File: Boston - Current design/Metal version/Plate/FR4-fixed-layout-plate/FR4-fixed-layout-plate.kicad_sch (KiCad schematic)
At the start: 14 parts

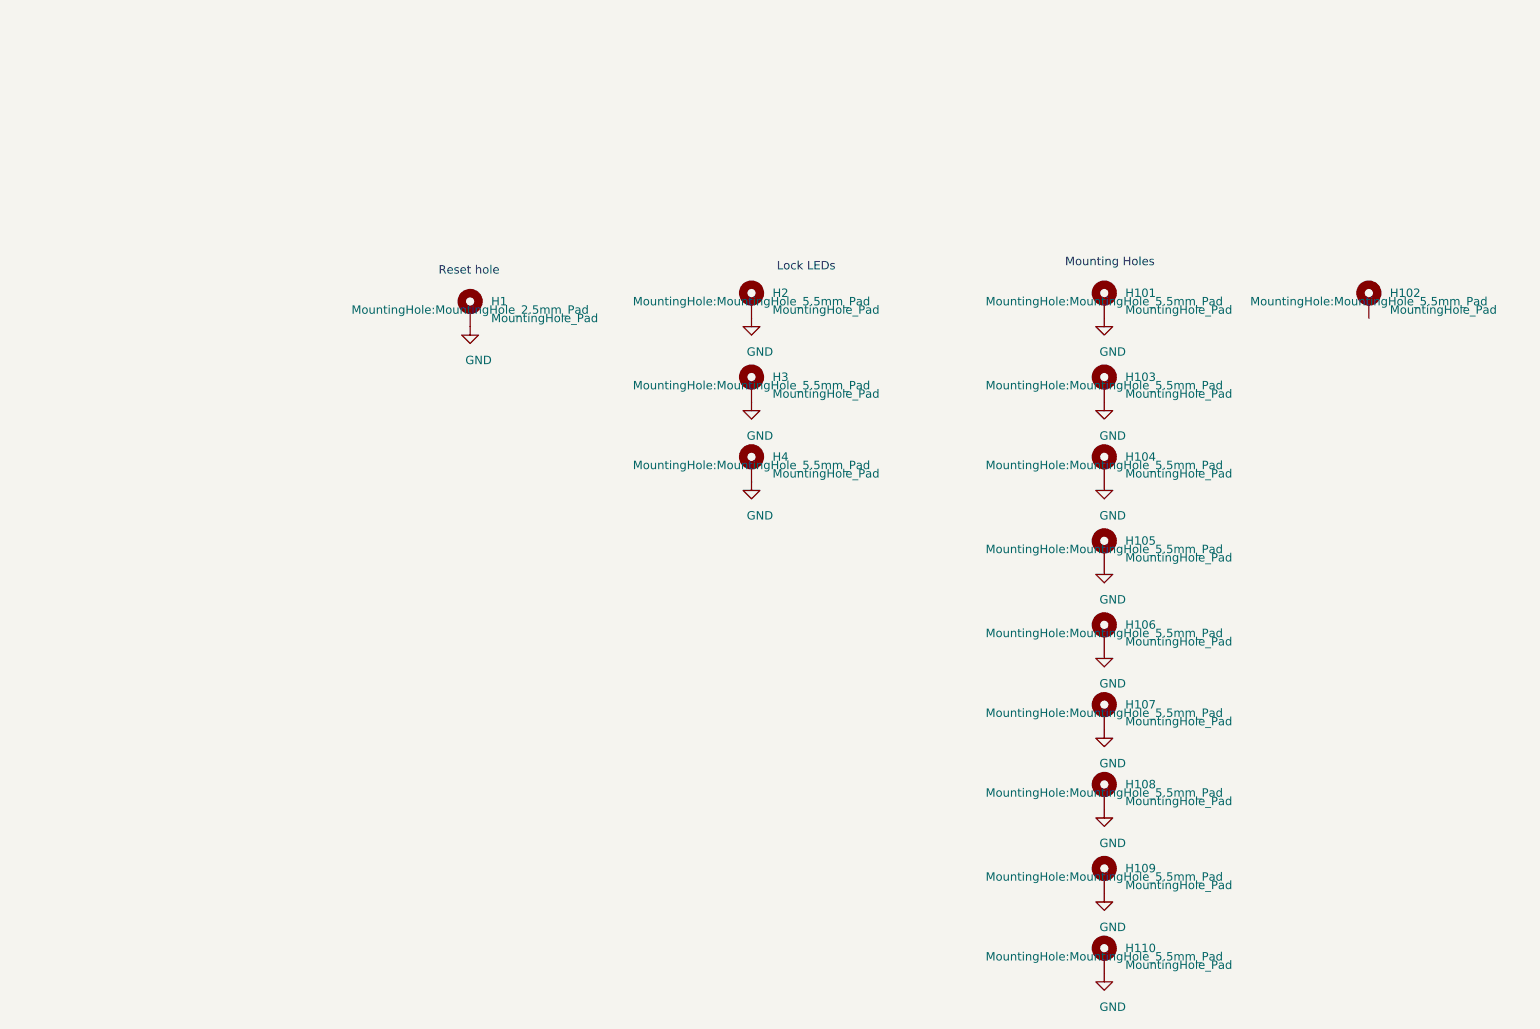
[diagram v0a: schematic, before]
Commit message: Finished work on fixed layout plate
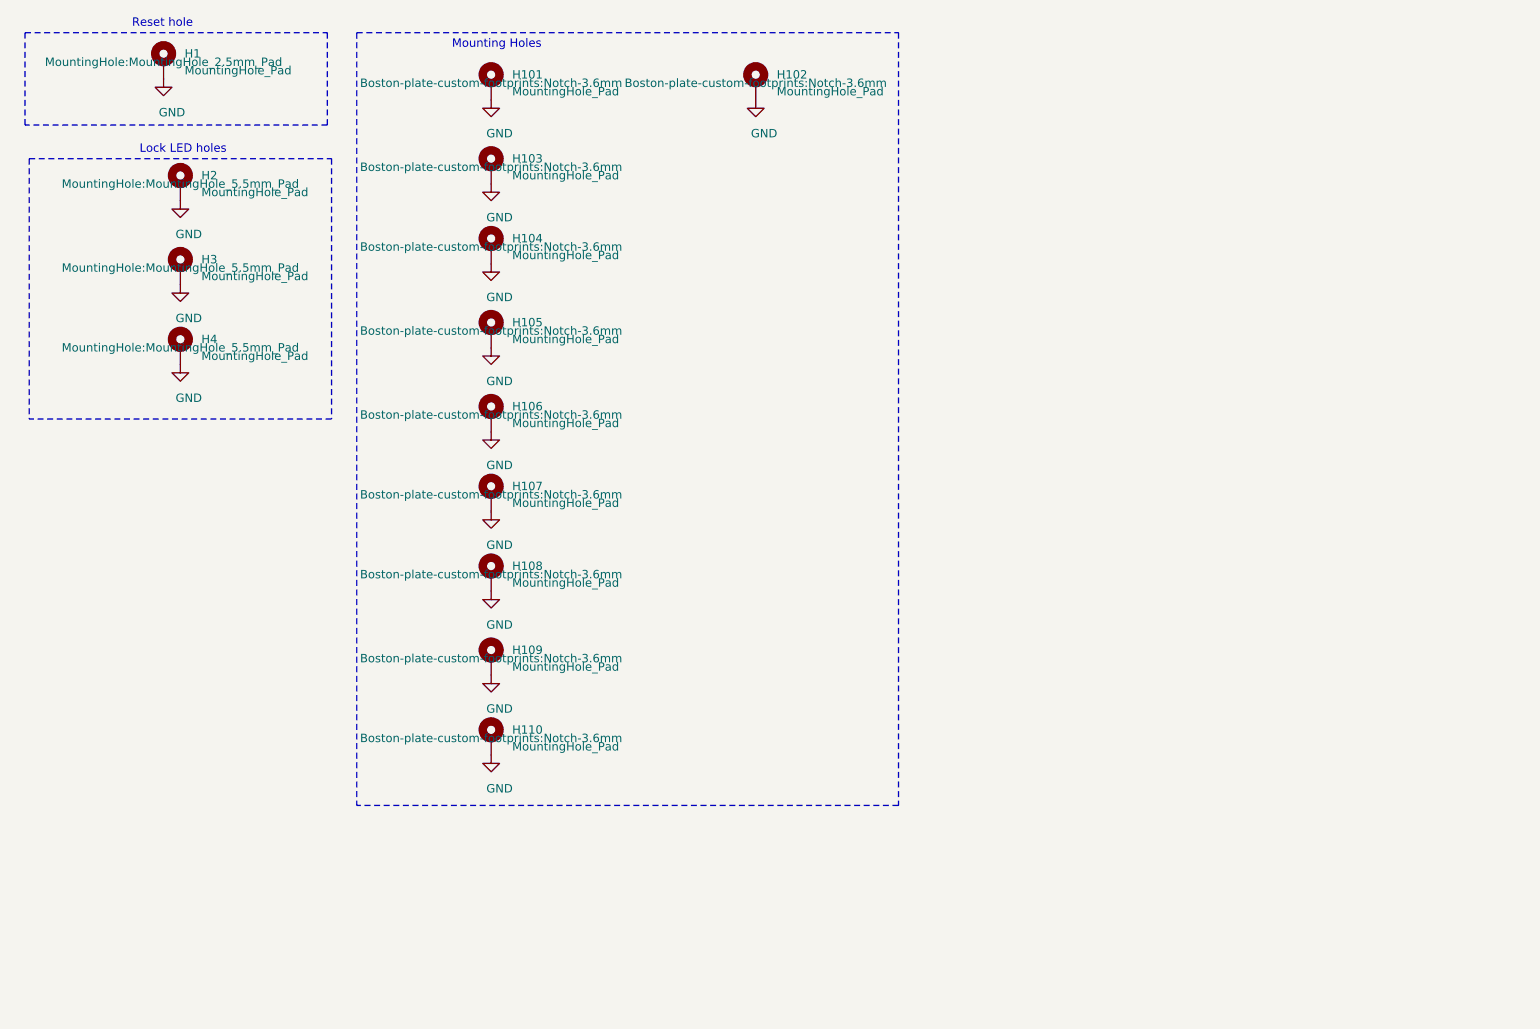
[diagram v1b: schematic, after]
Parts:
- H101, H102, H103, H104, H105, H106, H107, H108, H109, H110: footprint MountingHole:MountingHole_5.5mm_Pad -> Boston-plate-custom-footprints:Notch-3.6mm
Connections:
- net GND: now also H102.1
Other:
- note added: "Lock LED holes"
- note removed: "Lock LEDs"
- moved on the sheet: H1, H101, H102, H103, H104, H105, H106, H107, H108, H109, H110, H2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
